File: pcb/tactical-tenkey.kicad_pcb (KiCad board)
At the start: 2 copper layers, 45 parts, among them J1 io_side, J2 esp32_side, J3 OLED, Q1 FS8205A, SW1 SW_SPST, U1 XIAO-ESP32-S3-SMD, U2 DW01A

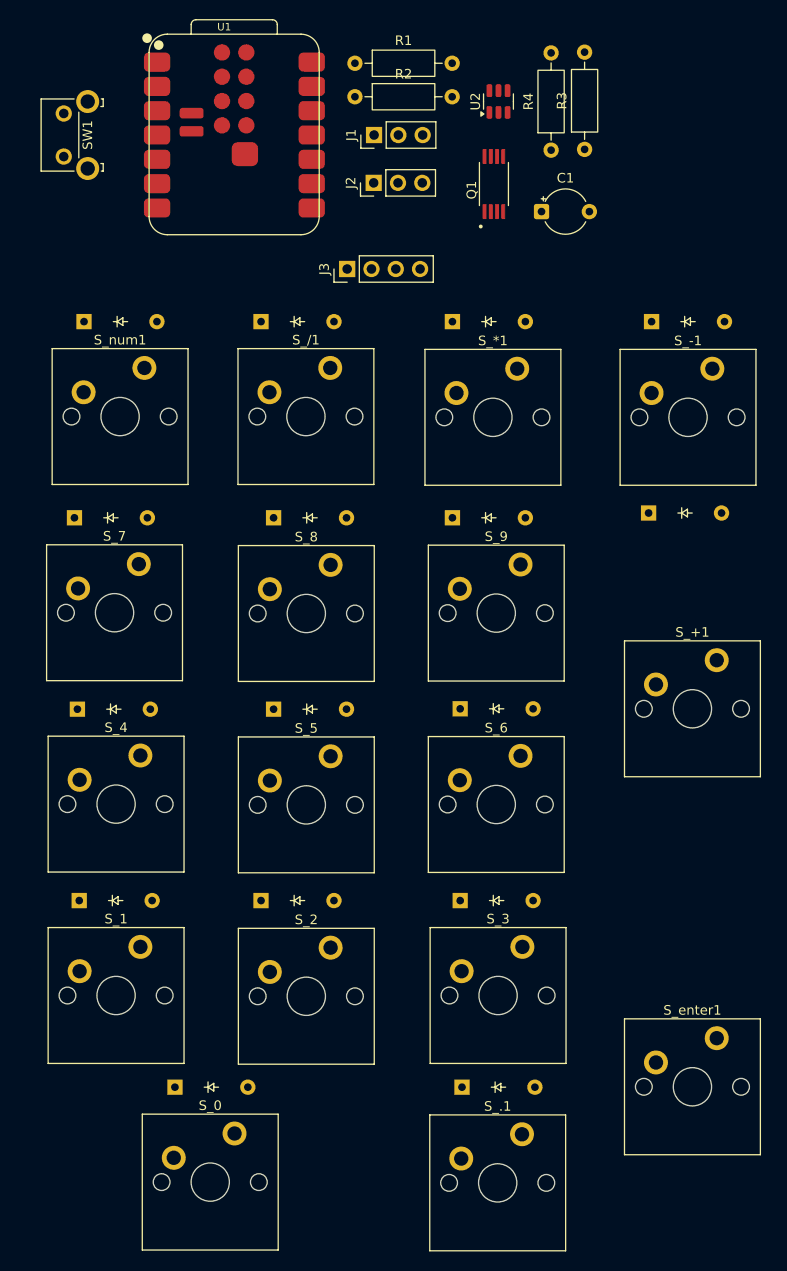
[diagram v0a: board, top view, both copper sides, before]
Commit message: routing
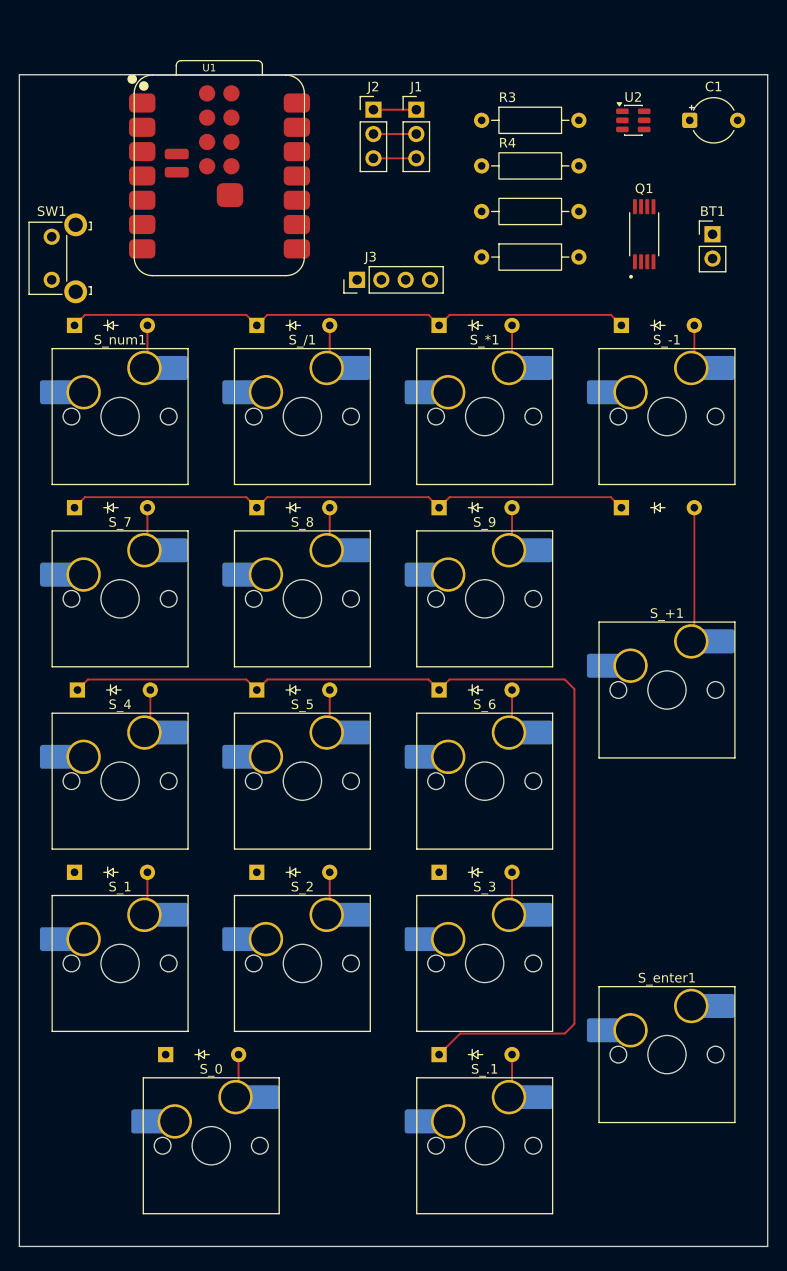
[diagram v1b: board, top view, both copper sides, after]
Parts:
- added BT1: 18650, Connector_PinHeader_2.54mm:PinHeader_1x02_P2.54mm_Vertical, F.Cu at (141.4, 55.9)
- S_*1, S_-1, S_.1, S_/1, S_1, S_2, S_3, S_4, S_5, S_6, S_7, S_8, S_9: footprint ScottoKeebs_MX:MX_PCB_1.00u -> ScottoKeebs_Hotswap:Hotswap_MX_Plated_1.00u
- S_+1, S_enter1: footprint ScottoKeebs_MX:MX_PCB_2.00u_90deg -> ScottoKeebs_Hotswap:Hotswap_MX_Plated_2.00u_90deg
- S_0: footprint ScottoKeebs_MX:MX_PCB_2.00u -> ScottoKeebs_Hotswap:Hotswap_MX_Plated_2.00u
- S_num1: footprint ScottoKeebs_MX:MX_PCB -> ScottoKeebs_Hotswap:Hotswap_MX_Plated_1.00u
- U1: footprint xiao:XIAO-ESP32-S3-SMD_PAD -> Seeed_Studio_XIAO_Series:XIAO-ESP32-S3-SMD_PAD
- moved R1 28.1 mm to (127.4, 53.5), turned to 180 degrees
- moved R2 21.4 mm to (117.2, 58.3)
- moved C1 18.2 mm to (139.0, 44.0)
- moved Q1 16.6 mm to (134.2, 55.9)
- moved U2 14.2 mm to (133.1, 44.0), turned to 0 degrees
- moved SW1 12.9 mm to (72.3, 60.6)
- moved R3 11.2 mm to (117.2, 44.0), turned to 0 degrees
- moved J2 7.65 mm to (105.9, 42.9), turned to 0 degrees
- moved J1 5.15 mm to (110.4, 42.9), turned to 0 degrees
- moved U1 4.55 mm to (80.9, 60.3)
- moved S_enter1 4.29 mm to (136.6, 141.6)
- moved D14 4.16 mm to (112.8, 141.6)
- moved S_.1 4.11 mm to (117.6, 151.1)
- moved S_0 3.80 mm to (89.0, 151.1)
- moved D13 3.69 mm to (112.8, 122.5)
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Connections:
- J2 pad 1: Net-(J2-Pin_1) -> row_1
- J2 pad 2: Net-(J2-Pin_2) -> Net-(J1-Pin_2)
- J2 pad 3: Net-(J2-Pin_3) -> pwr
- R1 pad 1: Net-(J1-Pin_2) -> prot+
- R1 pad 2: +BATT -> Net-(J1-Pin_2)
- R2 pad 1: -BATT -> Net-(J1-Pin_2)
- R2 pad 2: Net-(J1-Pin_2) -> GND
- R4 pad 1: GND -> Net-(U2-CS)
- R4 pad 2: Net-(U2-CS) -> GND
- U1 pad 1: Net-(J2-Pin_3) -> pwr
- U1 pad 15: (no net) -> prot+
- U1 pad 16: (no net) -> unconnected-(U1-GND-Pad16)
- U1 pad 17: (no net) -> unconnected-(U1-GPIO41_MTDI-Pad17)
- U1 pad 18: (no net) -> unconnected-(U1-GPIO40_MTDO-Pad18)
- U1 pad 19: (no net) -> unconnected-(U1-CHIP_EN-Pad19)
- U1 pad 20: (no net) -> unconnected-(U1-GND-Pad20)
- U1 pad 21: (no net) -> row_1
- U1 pad 22: (no net) -> unconnected-(U1-GPIO39_MTCK-Pad22)
- U1 pad 23: (no net) -> unconnected-(U1-GPIO19_USB_DN-Pad23)
- U1 pad 3: Net-(J2-Pin_2) -> Net-(J1-Pin_2)
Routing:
- net row_3: track 0.00 -> 105.1 mm
- net row_1: track 0.00 -> 64.4 mm
- net row_2: track 0.00 -> 59.9 mm
- net Net-(D16-A): track 0.00 -> 14.1 mm
- net Net-(D8-A): track 0.00 -> 4.70 mm
- net Net-(D7-A): track 0.00 -> 4.58 mm
- net Net-(D6-A): track 0.00 -> 4.58 mm
- net Net-(D3-A): track 0.00 -> 4.58 mm
- net Net-(D2-A): track 0.00 -> 4.58 mm
- net Net-(D5-A): track 0.00 -> 4.58 mm
- net Net-(D9-A): track 0.00 -> 4.58 mm
- net Net-(D4-A): track 0.00 -> 4.58 mm
- net Net-(D14-A): track 0.00 -> 4.58 mm
- net Net-(D13-A): track 0.00 -> 4.58 mm
- net Net-(D12-A): track 0.00 -> 4.58 mm
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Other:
- board outline added: 78.2 x 122.4 mm

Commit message: case
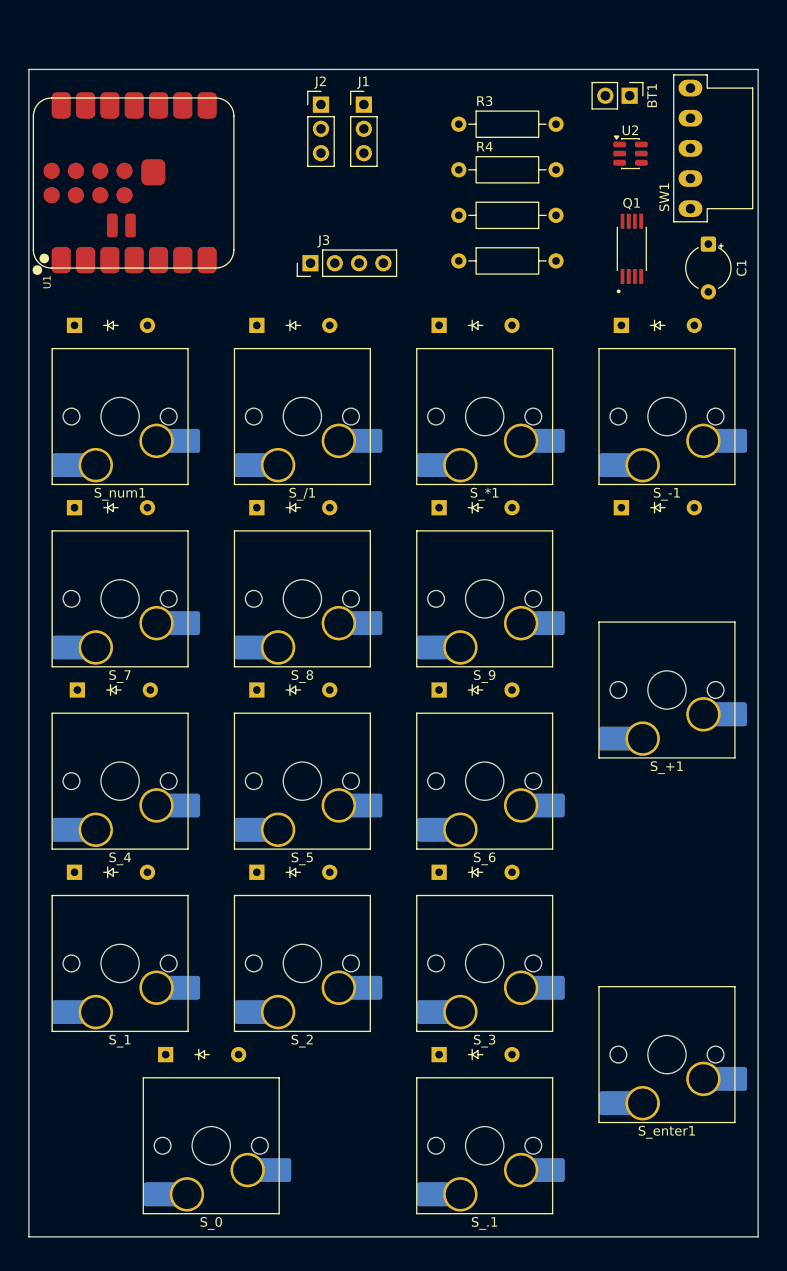
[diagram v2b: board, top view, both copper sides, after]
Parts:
- SW1: value SW_SPST -> SW_SPDT; footprint Button_Switch_THT:SW_SPST_Omron_B3F-315x_Angled -> Personal:SS-12F23G5
- U1: footprint Seeed_Studio_XIAO_Series:XIAO-ESP32-S3-SMD_PAD -> xiao:XIAO-ESP32-S3-SMD_PAD
- moved SW1 68.1 mm to (139.1, 46.9)
- moved BT1 16.9 mm to (132.7, 41.4), turned to -90 degrees
- moved C1 13.1 mm to (140.9, 56.9), turned to -90 degrees
- moved U1 10.5 mm to (91.4, 59.4), turned to 90 degrees
- moved J1 5.51 mm to (104.9, 42.3)
- moved J2 5.51 mm to (100.5, 42.3)
- moved J3 5.17 mm to (99.4, 58.9)
- moved U2 3.49 mm to (132.8, 47.4)
- moved R1 2.42 mm to (125.0, 53.9)
- moved R2 2.42 mm to (114.9, 58.7)
- moved R3 2.42 mm to (114.9, 44.4)
- moved R4 2.42 mm to (125.0, 49.1)
- moved Q1 2.00 mm to (132.9, 57.4)
- turned S_*1 to 180 degrees
- turned S_+1 to 180 degrees
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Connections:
- SW1 pad 1: +BATT -> prot+
- SW1 pad 2: prot+ -> +BATT
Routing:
- net row_3: track 105.1 -> 0.00 mm
- net row_1: track 64.4 -> 0.00 mm
- net row_2: track 59.9 -> 0.00 mm
- net Net-(D16-A): track 14.1 -> 0.00 mm
- net Net-(D8-A): track 4.70 -> 0.00 mm
- net Net-(D7-A): track 4.58 -> 0.00 mm
- net Net-(D6-A): track 4.58 -> 0.00 mm
- net Net-(D3-A): track 4.58 -> 0.00 mm
- net Net-(D2-A): track 4.58 -> 0.00 mm
- net Net-(D5-A): track 4.58 -> 0.00 mm
- net Net-(D9-A): track 4.58 -> 0.00 mm
- net Net-(D4-A): track 4.58 -> 0.00 mm
- net Net-(D14-A): track 4.58 -> 0.00 mm
- net Net-(D13-A): track 4.58 -> 0.00 mm
- net Net-(D12-A): track 4.58 -> 0.00 mm
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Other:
- board size 78.2 x 122.4 mm -> 76.2 x 122 mm
